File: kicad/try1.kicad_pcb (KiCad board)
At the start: 2 copper layers, 83.8 x 68.6 mm, 113 parts, among them J1 Conn_02x11_Odd_Even, J2 Conn_01x08_Female, J3 Conn_01x03, J4 USB_A, J5 USB_B_Micro, SW1 LL3301NF065QG-proy, SW2 LL3301NF065QG-proy, U1 ICE40UP5K-SG48ITR50-proy, U10 ZLDO1117G33TA-proy, U2 AD7918BRUZ-proy, U3 W25Q32JVSS-proy, U4 STM32F100RBT6B-proy, U5 Omega2-proy, U6 ZLDO1117G12TA-proy, U7 ZLDO1117G25TA-proy, U8 ZLDO1117G33TA-proy, U9 ZLDO1117G33TA-proy, X1 CWX823-025.0M-proy

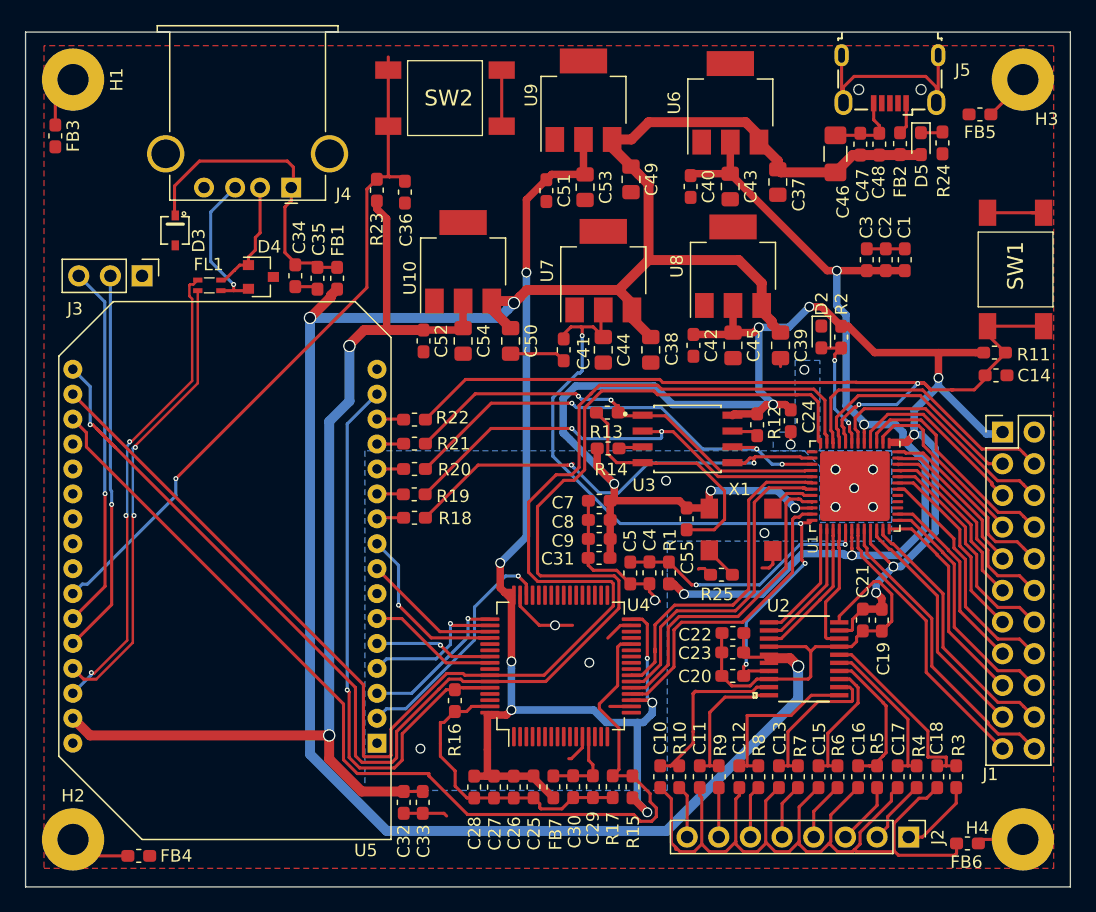
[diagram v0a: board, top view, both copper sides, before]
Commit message: Add files via upload
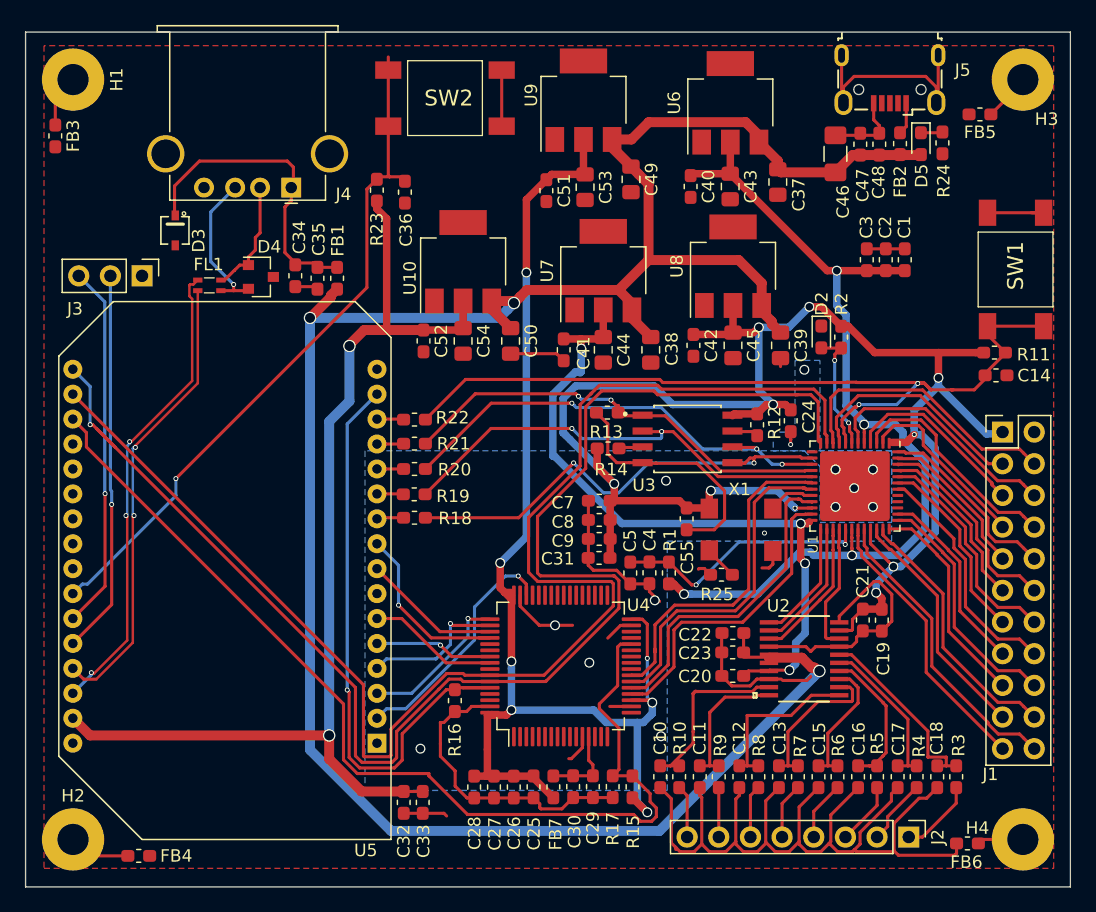
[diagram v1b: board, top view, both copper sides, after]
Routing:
- net +2.5V_FPGA: track 57.4 -> 63.9 mm
- net GND: track 224.2 -> 222.2 mm, vias 13 -> 14
- net +5V: track 194.3 -> 195.7 mm
- net /FPGA_ICE40UP5K/I2C_FPGA_SCL: track 114.4 -> 113.7 mm
